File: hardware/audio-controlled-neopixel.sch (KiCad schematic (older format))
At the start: 64 parts, among them J1 AudioJack4, J2 AudioJack4, J3 KF2EDGK, J4 KF2EDGK, J5 KF2EDGK, J6 Conn_01x01_Female, J7 Conn_01x01_Female, J8 Conn_01x01_Female, J9 Conn_01x01_Female, SW1 SW_SPST, U1 LM324, U2 TMA0512D, U3 LM324

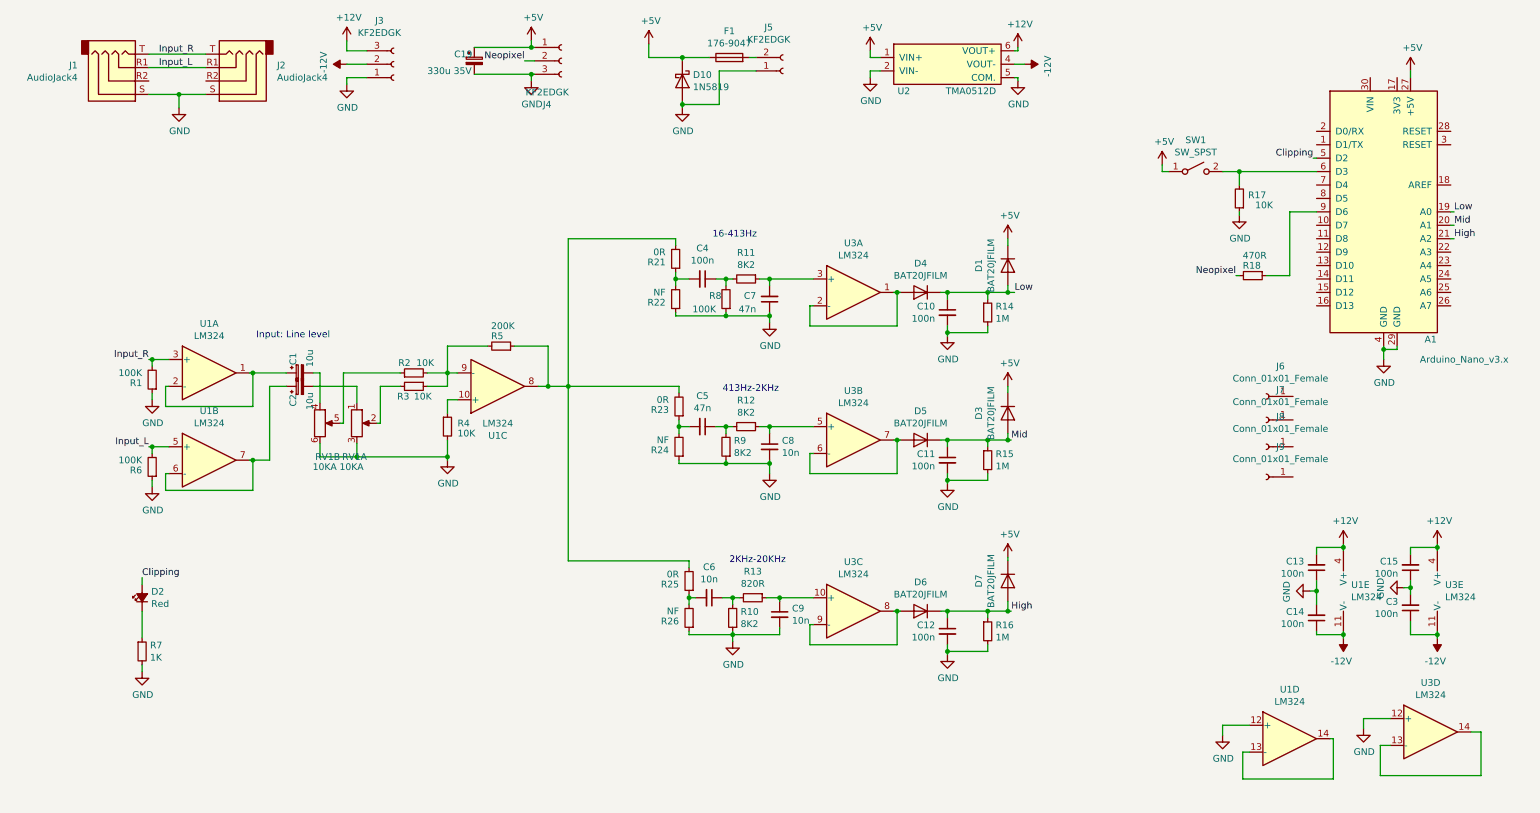
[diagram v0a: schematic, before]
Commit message: hardware updates
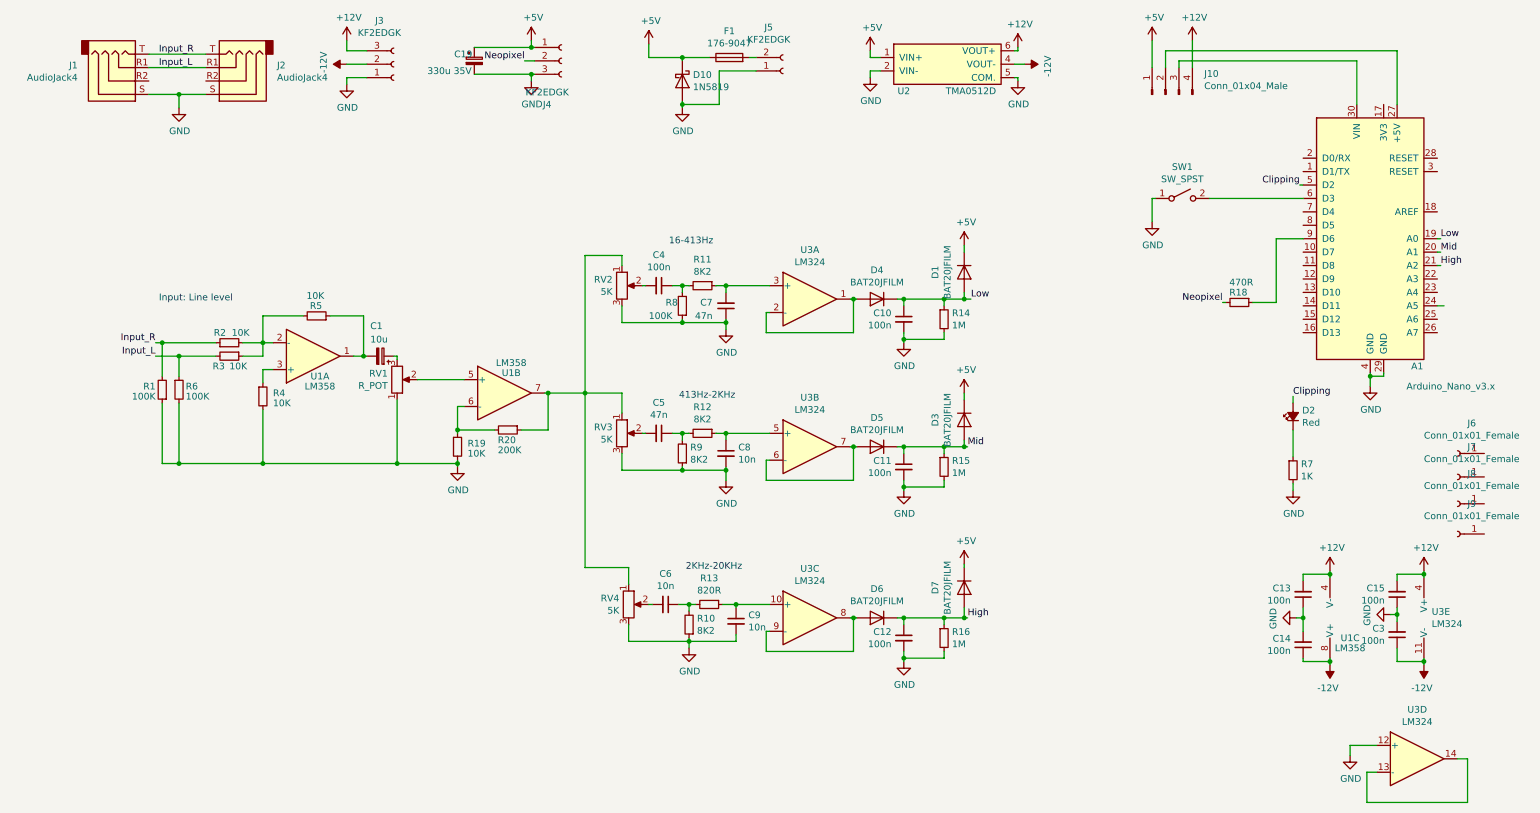
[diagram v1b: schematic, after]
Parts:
- removed C2: 10u, Capacitor_THT:CP_Radial_D5.0mm_P2.00mm, symbol Device:CP_Small
- removed R17: 10K, Resistor_SMD:R_0805_2012Metric, symbol Device:R_Small
- removed R21, R23, R25: 0R, Resistor_SMD:R_0805_2012Metric, symbol Device:R_Small
- removed R22, R24, R26: NF, Resistor_SMD:R_0805_2012Metric, symbol Device:R_Small
- removed RV1: 10KA, Potentiometer_THT:Potentiometer_Alps_RK097_Dual_Horizontal, symbol Device:R_POT_Dual_Separate
- removed U1: LM324, Package_SO:SOIC-14_3.9x8.7mm_P1.27mm, symbol Amplifier_Operational:LM324
- added J10: Conn_01x04_Male, Connector_PinHeader_2.54mm:PinHeader_1x04_P2.54mm_Vertical, symbol Connector:Conn_01x04_Male
- added R19: 10K, Resistor_SMD:R_0805_2012Metric, symbol Device:R_Small
- added R20: 200K, Resistor_SMD:R_0805_2012Metric, symbol Device:R_Small
- added RV1: R_POT, Potentiometer_THT:Potentiometer_Alps_RK097_Single_Horizontal, symbol Device:R_POT
- added RV2, RV3, RV4: 5K, Potentiometer_SMD:Potentiometer_Vishay_TS53YJ_Vertical, symbol Device:R_POT
- added U1: LM358, Package_SO:SOIC-8_3.9x4.9mm_P1.27mm, symbol Amplifier_Operational:LM358
- C19: footprint Capacitor_THT:CP_Radial_D10.0mm_P5.00mm -> Capacitor_SMD:CP_Elec_10x10
- J1, J2: footprint Connector_Audio:Jack_3.5mm_PJ320D_Horizontal -> custom:Jack_3.5mm_PJ320D_Horizontal
- R5: value 200K -> 10K
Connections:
- net +12V: now also J10.4 (Pin_4), U1.4 (V-)
- net +5V: now also J10.1 (Pin_1); no longer A1.27 (+5V), SW1.1 (A)
- net -12V: now also U1.8 (V+)
- net GND: now also R6.2, SW1.1 (A), R19.2, RV1.1, RV2.3, RV3.3, RV4.3; no longer R6.1
- net Input_L: now also R3.2, R6.1; no longer R6.2
- net Input_R: now also R2.1
- net at C6.2: now also RV4.2
- net at C5.2: now also RV3.2
- net at R2.2, R3.1, R5.2: now also U1.2 (-)
- net at R5.1: now also C1.2, U1.1
- net at C4.2: now also RV2.2
- net at R4.1: now also U1.3 (+)
- net at A1.30 (VIN): now also J10.3 (Pin_3)
- net at C1.1: now also RV1.3
- new net: A1.27 (+5V), J10.2 (Pin_2)
- new net: RV1.2, U1.5 (+)
- new net: R19.1, R20.2, U1.6 (-)
- new net: R20.1, RV2.1, RV3.1, RV4.1, U1.7
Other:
- moved on the sheet: A1, C1, C10, C11, C12, C13, C14, C15, C3, C4, C5, C6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
